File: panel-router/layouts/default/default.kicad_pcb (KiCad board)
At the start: 2 copper layers, 21 x 94 mm, 4 parts

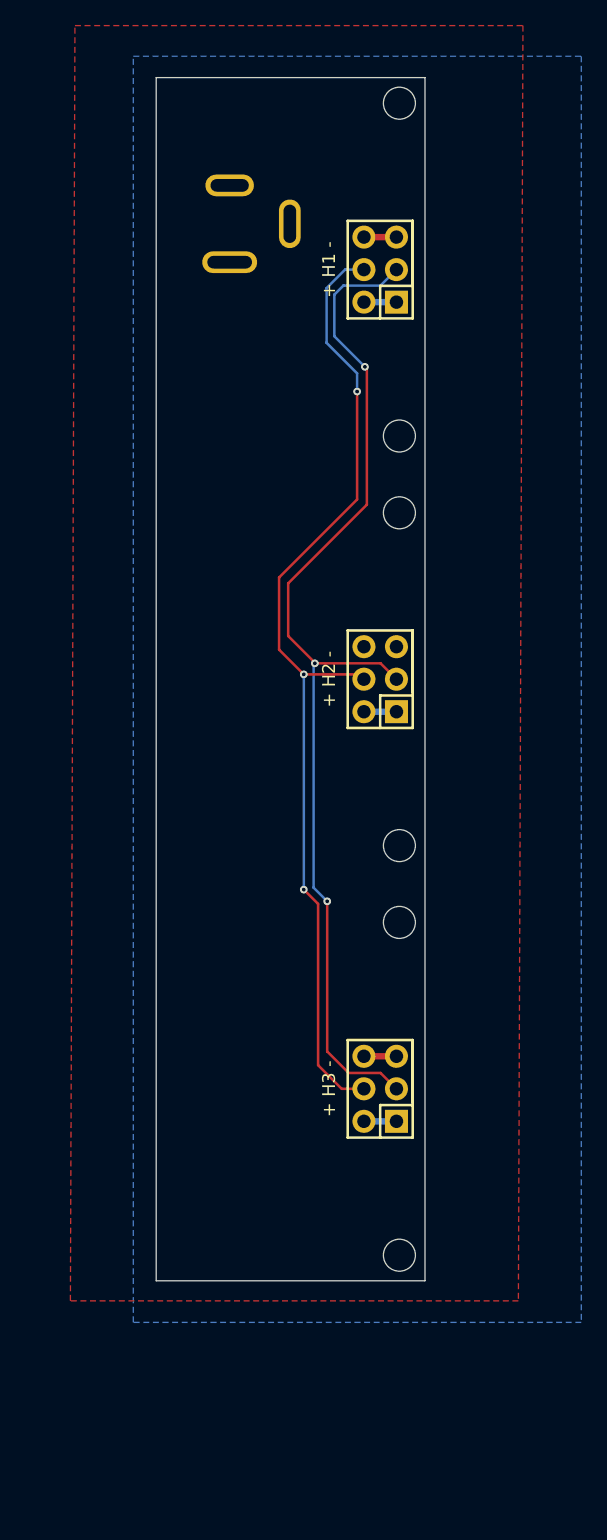
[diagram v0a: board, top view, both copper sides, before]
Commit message: Header & Silkscreen Updates
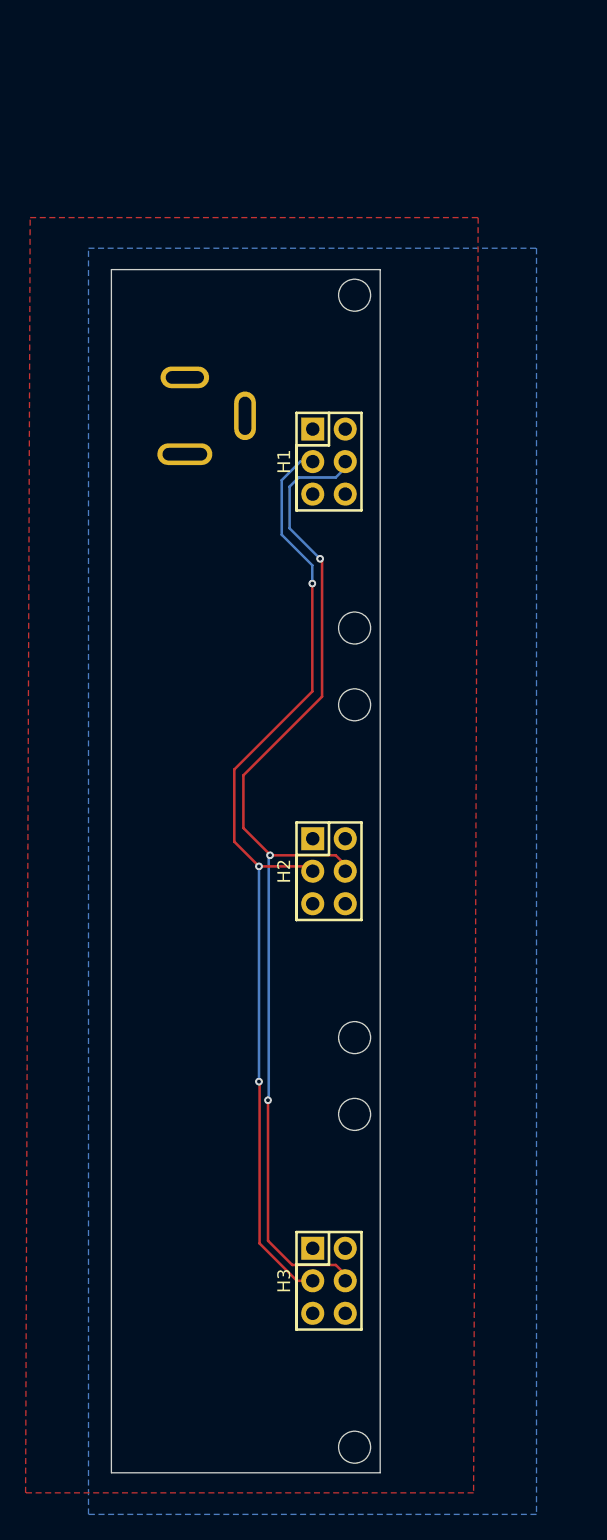
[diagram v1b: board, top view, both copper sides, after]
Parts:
- H1: renamed from + H1 -
- H2: renamed from + H2 -
- H3: renamed from + H3 -
- moved H1 15.5 mm to (96.0, 115.0), turned to -90 degrees
- moved H2 15.5 mm to (96.0, 147.0), turned to -90 degrees
- moved H3 15.5 mm to (96.0, 179.0), turned to -90 degrees
- moved 15V-25V DC 15.4 mm to (87.1, 111.4)
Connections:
- H1 pad 2: V+ -> GND
- H1 pad 5: GND -> V+
- H2 pad 2: V+ -> GND
- H2 pad 5: GND -> V+
- H3 pad 2: V+ -> GND
- H3 pad 5: GND -> V+
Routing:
- net V+: track 7.62 -> 0.00 mm
- net 4: track 78.2 -> 83.8 mm
- net GND: track 5.08 -> 0.00 mm
- net 3: track 83.2 -> 78.2 mm

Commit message: Basic layout tweaks
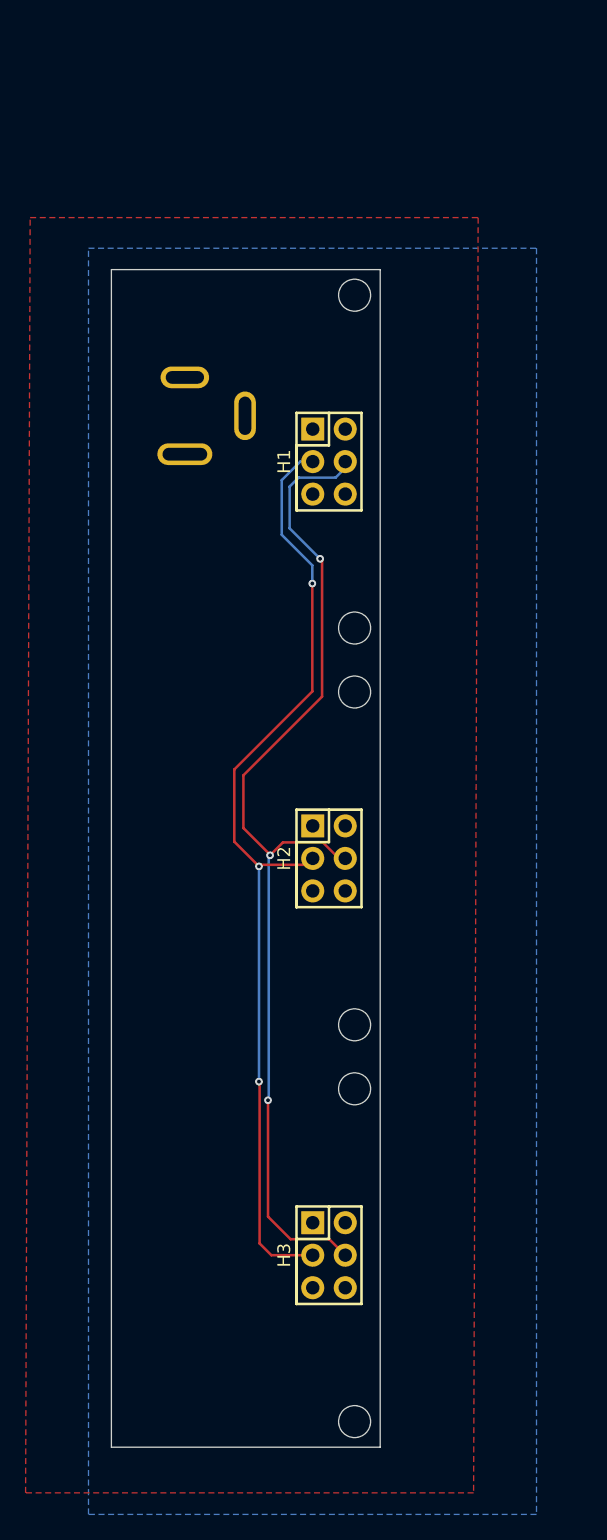
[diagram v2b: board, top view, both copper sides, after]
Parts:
- moved H3 2.00 mm to (96.0, 177.0)
- moved H2 1.00 mm to (96.0, 146.0)
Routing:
- net 4: track 83.8 -> 81.3 mm
- net 3: track 78.2 -> 77.2 mm
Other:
- board size 21 x 94 mm -> 21 x 92 mm
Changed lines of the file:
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@@
 	(footprint "BOOMELE_2_54_2_3P:HDR-TH_6P-P2.54-V-M-R2-C3-S2.54-1"
 		(layer "F.Cu")
-		(at 96 147 -90)
+		(at 96 146 -90)
 		(property "Reference" "H2"
 			(at 0 3.5 90)
@@
 	(footprint "BOOMELE_2_54_2_3P:HDR-TH_6P-P2.54-V-M-R2-C3-S2.54-1"
 		(layer "F.Cu")
-		(at 96 179 -90)
+		(at 96 177 -90)
 		(property "Reference" "H3"
 			(at 0 3.5 90)
@@
 	)
 	(gr_circle
-		(center 98 134)
-		(end 99.25 134)
+		(center 98 133)
+		(end 99.25 133)
 		(stroke
 			(width 0.05)
@@
 	)
 	(gr_circle
-		(center 98 160)
-		(end 99.25 160)
+		(center 98 159)
+		(end 99.25 159)
 		(stroke
 			(width 0.05)
@@
 	(gr_rect
 		(start 79 100)
-		(end 100 194)
+		(end 100 192)
 		(stroke
 			(width 0.05)
@@
 	)
 	(gr_circle
-		(center 98 192)
-		(end 99.25 192)
+		(center 98 190)
+		(end 99.25 190)
 		(stroke
 			(width 0.05)
@@
 	)
 	(gr_circle
-		(center 98 166)
-		(end 99.25 166)
+		(center 98 164)
+		(end 99.25 164)
 		(stroke
 			(width 0.05)
@@
 	)
 	(segment
-		(start 94.8528 146.6228)
-		(end 95.23 147)
-		(width 0.2)
-		(layer "F.Cu")
-		(net 1)
-	)
-	(segment
 		(start 90.5308 146.6228)
 		(end 88.6004 144.6924)
@@
 	)
 	(segment
+		(start 94.73 177)
+		(end 95.23 177.5)
+		(width 0.2)
+		(layer "F.Cu")
+		(net 1)
+	)
+	(segment
 		(start 90.5764 163.4832)
 		(end 90.5764 176.0816)
@@
 	)
 	(segment
+		(start 90.5308 146.6228)
+		(end 90.6536 146.5)
+		(width 0.2)
+		(layer "F.Cu")
+		(net 1)
+	)
+	(segment
+		(start 94.6964 132.9576)
+		(end 94.6964 124.5248)
+		(width 0.2)
+		(layer "F.Cu")
+		(net 1)
+	)
+	(segment
+		(start 94.23 146.5)
+		(end 94.73 146)
+		(width 0.2)
+		(layer "F.Cu")
+		(net 1)
+	)
+	(segment
 		(start 90.5308 163.4376)
 		(end 90.5764 163.4832)
@@
 	)
 	(segment
-		(start 94.6964 132.9576)
-		(end 94.6964 124.5248)
-		(width 0.2)
-		(layer "F.Cu")
-		(net 1)
-	)
-	(segment
-		(start 93.4948 179)
-		(end 95.23 179)
-		(width 0.2)
-		(layer "F.Cu")
-		(net 1)
-	)
-	(segment
-		(start 90.5308 146.6228)
-		(end 94.8528 146.6228)
-		(width 0.2)
-		(layer "F.Cu")
-		(net 1)
-	)
-	(segment
 		(start 90.5764 176.0816)
-		(end 93.4948 179)
+		(end 91.4948 177)
+		(width 0.2)
+		(layer "F.Cu")
+		(net 1)
+	)
+	(segment
+		(start 91.4948 177)
+		(end 94.73 177)
+		(width 0.2)
+		(layer "F.Cu")
+		(net 1)
+	)
+	(segment
+		(start 90.6536 146.5)
+		(end 94.23 146.5)
 		(width 0.2)
 		(layer "F.Cu")
@@
 	)
 	(segment
+		(start 96.77 146)
+		(end 97.27 146)
+		(width 0.2)
+		(layer "F.Cu")
+		(net 2)
+	)
+	(segment
 		(start 89.3116 143.6256)
 		(end 89.3116 139.5108)
@@
 	)
 	(segment
+		(start 91.2368 173.9868)
+		(end 93 175.75)
+		(width 0.2)
+		(layer "F.Cu")
+		(net 2)
+	)
+	(segment
 		(start 95.4584 133.364)
 		(end 95.4584 122.7468)
@@
 	)
 	(segment
-		(start 96.5332 177.7632)
-		(end 97.77 179)
+		(start 96.02 175.75)
+		(end 97.27 177)
 		(width 0.2)
 		(layer "F.Cu")
@@
 	)
 	(segment
-		(start 93.1304 177.7632)
-		(end 96.5332 177.7632)
+		(start 92.4036 144.75)
+		(end 95.52 144.75)
 		(width 0.2)
 		(layer "F.Cu")
@@
 	)
 	(segment
-		(start 96.5292 145.7592)
-		(end 97.77 147)
+		(start 91.3944 145.7592)
+		(end 92.4036 144.75)
 		(width 0.2)
 		(layer "F.Cu")
@@
 	)
 	(segment
-		(start 91.2368 175.8696)
-		(end 93.1304 177.7632)
-		(width 0.2)
-		(layer "F.Cu")
-		(net 2)
-	)
-	(segment
 		(start 91.2928 145.6576)
 		(end 91.2928 145.6068)
@@
 	)
 	(segment
+		(start 95.52 144.75)
+		(end 96.77 146)
+		(width 0.2)
+		(layer "F.Cu")
+		(net 2)
+	)
+	(segment
 		(start 91.2368 164.8968)
-		(end 91.2368 175.8696)
-		(width 0.2)
-		(layer "F.Cu")
-		(net 2)
-	)
-	(segment
-		(start 91.3944 145.7592)
-		(end 96.5292 145.7592)
+		(end 91.2368 173.9868)
 		(width 0.2)
 		(layer "F.Cu")
@@
 		(width 0.2)
 		(layer "F.Cu")
+		(net 2)
+	)
+	(segment
+		(start 93 175.75)
+		(end 96.02 175.75)
+		(width 0.2)
+		(layer "F.Cu")
